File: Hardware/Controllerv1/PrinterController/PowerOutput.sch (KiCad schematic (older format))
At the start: 33 parts, among them J3 Conn_01x03, J4 Conn_01x03, J5 Screw_Terminal_01x08, Q1 Q_NMOS_DGS, Q2 Q_NMOS_DGS, Q3 Q_NMOS_DGS, Q4 Q_NMOS_DGS, Q5 Q_NMOS_DGS, Q6 Q_NMOS_DGS, U2 ZXGD3003E6, U3 ZXGD3003E6, U4 ZXGD3003E6, U5 ZXGD3003E6, U6 ZXGD3003E6, U7 ZXGD3003E6

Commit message: Added updates to PCB
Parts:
- removed Q1, Q2, Q3, Q4: Q_NMOS_DGS, .pretty:SOT65P330X90-5N, symbol Q_NMOS_DGS
- added U10, U11, U8, U9: IRFR3711TRPBF, IRFR3711TRPBF:TO252, symbol IRFR3711TRPBF
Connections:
- net labels removed: VDC
- wire segments 75 -> 81

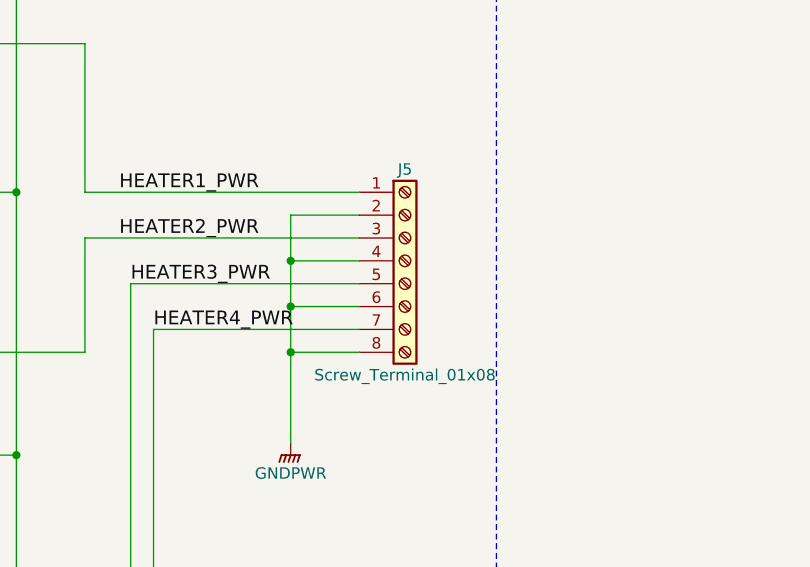
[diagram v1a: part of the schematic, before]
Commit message: Updated PCBS
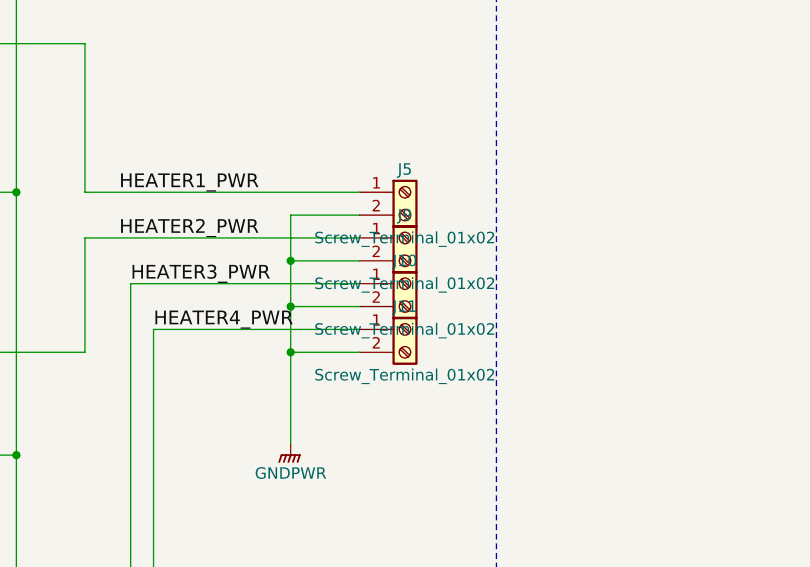
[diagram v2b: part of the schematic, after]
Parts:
- removed J5: Screw_Terminal_01x08, TerminalBlocks_WAGO:TerminalBlock_WAGO-804_RM5mm_8pol, symbol Screw_Terminal_01x08
- added J10, J11, J5, J9: Screw_Terminal_01x02, TerminalBlocks_Phoenix:TerminalBlock_Phoenix_PT-3.5mm_2pol, symbol Screw_Terminal_01x02
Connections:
- net GNDPWR: now also J10.2 (Pin_2), J11.2 (Pin_2), J5.2 (Pin_2), J9.2 (Pin_2)
- net HEATER1_PWR: now also J5.1 (Pin_1)
- net HEATER2_PWR: now also J9.1 (Pin_1)
- net HEATER3_PWR: now also J10.1 (Pin_1)
- net HEATER4_PWR: now also J11.1 (Pin_1)
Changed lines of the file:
@@
 Connection ~ 4050 2450
 $Comp
-L +VDC #PWR077
+L +VDC #PWR083
 U 1 1 5B23E478
 P 4050 1350
-F 0 "#PWR077" H 4050 1250 50  0001 C CNN
+F 0 "#PWR083" H 4050 1250 50  0001 C CNN
 F 1 "+VDC" H 4050 1600 50  0000 C CNN
 F 2 "" H 4050 1350 50  0001 C CNN
@@
 $EndComp
 $Comp
-L Screw_Terminal_01x08 J5
-U 1 1 5B23E5D0
-P 5750 2750
-F 0 "J5" H 5750 3150 50  0000 C CNN
-F 1 "Screw_Terminal_01x08" H 5750 2250 50  0000 C CNN
-F 2 "TerminalBlocks_WAGO:TerminalBlock_WAGO-804_RM5mm_8pol" H 5750 2750 50  0001 C CNN
-F 3 "" H 5750 2750 50  0001 C CNN
-	1    5750 2750
-	1    0    0    -1
-$EndComp
-$Comp
-L GND #PWR078
+L GND #PWR084
 U 1 1 5B23EDD4
 P 2150 1850
-F 0 "#PWR078" H 2150 1600 50  0001 C CNN
+F 0 "#PWR084" H 2150 1600 50  0001 C CNN
 F 1 "GND" H 2150 1700 50  0000 C CNN
 F 2 "" H 2150 1850 50  0001 C CNN
@@
 Connection ~ 4050 1350
 $Comp
-L GNDPWR #PWR079
+L GNDPWR #PWR085
 U 1 1 5B23F80C
 P 5250 3550
-F 0 "#PWR079" H 5250 3350 50  0001 C CNN
+F 0 "#PWR085" H 5250 3350 50  0001 C CNN
 F 1 "GNDPWR" H 5250 3420 50  0000 C CNN
 F 2 "" H 5250 3500 50  0001 C CNN
@@
 $EndComp
 $Comp
-L GND #PWR080
+L GND #PWR086
 U 1 1 5B240503
 P 2150 2950
-F 0 "#PWR080" H 2150 2700 50  0001 C CNN
+F 0 "#PWR086" H 2150 2700 50  0001 C CNN
 F 1 "GND" H 2150 2800 50  0000 C CNN
 F 2 "" H 2150 2950 50  0001 C CNN
@@
 $EndComp
 $Comp
-L GND #PWR081
+L GND #PWR087
 U 1 1 5B240680
 P 2200 4100
-F 0 "#PWR081" H 2200 3850 50  0001 C CNN
+F 0 "#PWR087" H 2200 3850 50  0001 C CNN
 F 1 "GND" H 2200 3950 50  0000 C CNN
 F 2 "" H 2200 4100 50  0001 C CNN
@@
 $EndComp
 $Comp
-L GND #PWR082
+L GND #PWR088
 U 1 1 5B2409DB
 P 2250 5250
-F 0 "#PWR082" H 2250 5000 50  0001 C CNN
+F 0 "#PWR088" H 2250 5000 50  0001 C CNN
 F 1 "GND" H 2250 5100 50  0000 C CNN
 F 2 "" H 2250 5250 50  0001 C CNN
@@
 	3500 6000 3500 6100
 $Comp
-L GNDPWR #PWR083
+L GNDPWR #PWR089
 U 1 1 5B24648A
 P 5050 5950
-F 0 "#PWR083" H 5050 5750 50  0001 C CNN
+F 0 "#PWR089" H 5050 5750 50  0001 C CNN
 F 1 "GNDPWR" H 5050 5820 50  0000 C CNN
 F 2 "" H 5050 5900 50  0001 C CNN
@@
 $EndComp
 $Comp
-L GNDPWR #PWR084
+L GNDPWR #PWR090
 U 1 1 5B246513
 P 5050 6700
-F 0 "#PWR084" H 5050 6500 50  0001 C CNN
+F 0 "#PWR090" H 5050 6500 50  0001 C CNN
 F 1 "GNDPWR" H 5050 6570 50  0000 C CNN
 F 2 "" H 5050 6650 50  0001 C CNN
@@
 $EndComp
 $Comp
-L GND #PWR085
+L GND #PWR091
 U 1 1 5B2466C8
 P 2250 6350
-F 0 "#PWR085" H 2250 6100 50  0001 C CNN
+F 0 "#PWR091" H 2250 6100 50  0001 C CNN
 F 1 "GND" H 2250 6200 50  0000 C CNN
 F 2 "" H 2250 6350 50  0001 C CNN
@@
 $EndComp
 $Comp
-L GND #PWR086
+L GND #PWR092
 U 1 1 5B2469E1
 P 2250 7450
-F 0 "#PWR086" H 2250 7200 50  0001 C CNN
+F 0 "#PWR092" H 2250 7200 50  0001 C CNN
 F 1 "GND" H 2250 7300 50  0000 C CNN
 F 2 "" H 2250 7450 50  0001 C CNN
@@
 	1700 3800 1700 3700
 $Comp
-L GND #PWR087
+L GND #PWR093
 U 1 1 5B248152
 P 6900 1300
-F 0 "#PWR087" H 6900 1050 50  0001 C CNN
+F 0 "#PWR093" H 6900 1050 50  0001 C CNN
 F 1 "GND" H 6900 1150 50  0000 C CNN
 F 2 "" H 6900 1300 50  0001 C CNN
@@
 $EndComp
 $Comp
-L GND #PWR088
+L GND #PWR094
 U 1 1 5B2481C7
 P 7200 1300
-F 0 "#PWR088" H 7200 1050 50  0001 C CNN
+F 0 "#PWR094" H 7200 1050 50  0001 C CNN
 F 1 "GND" H 7200 1150 50  0000 C CNN
 F 2 "" H 7200 1300 50  0001 C CNN
@@
 $EndComp
 $Comp
-L GND #PWR089
+L GND #PWR095
 U 1 1 5B248235
 P 7500 1300
-F 0 "#PWR089" H 7500 1050 50  0001 C CNN
+F 0 "#PWR095" H 7500 1050 50  0001 C CNN
 F 1 "GND" H 7500 1150 50  0000 C CNN
 F 2 "" H 7500 1300 50  0001 C CNN
@@
 $EndComp
 $Comp
-L GND #PWR090
+L GND #PWR096
 U 1 1 5B2482A3
 P 7800 1300
-F 0 "#PWR090" H 7800 1050 50  0001 C CNN
+F 0 "#PWR096" H 7800 1050 50  0001 C CNN
 F 1 "GND" H 7800 1150 50  0000 C CNN
 F 2 "" H 7800 1300 50  0001 C CNN
@@
 $EndComp
 $Comp
-L GND #PWR091
+L GND #PWR097
 U 1 1 5B248311
 P 8150 1300
-F 0 "#PWR091" H 8150 1050 50  0001 C CNN
+F 0 "#PWR097" H 8150 1050 50  0001 C CNN
 F 1 "GND" H 8150 1150 50  0000 C CNN
 F 2 "" H 8150 1300 50  0001 C CNN
@@
 $EndComp
 $Comp
-L GND #PWR092
+L GND #PWR098
 U 1 1 5B24837F
 P 8550 1300
-F 0 "#PWR092" H 8550 1050 50  0001 C CNN
+F 0 "#PWR098" H 8550 1050 50  0001 C CNN
 F 1 "GND" H 8550 1150 50  0000 C CNN
 F 2 "" H 8550 1300 50  0001 C CNN
@@
 	3600 1800 3600 1650
 $Comp
-L +VDC #PWR093
+L +VDC #PWR099
 U 1 1 5B262DD2
 P 6900 1000
-F 0 "#PWR093" H 6900 900 50  0001 C CNN
+F 0 "#PWR099" H 6900 900 50  0001 C CNN
 F 1 "+VDC" H 6900 1250 50  0000 C CNN
 F 2 "" H 6900 1000 50  0001 C CNN
@@
 $EndComp
 $Comp
-L +VDC #PWR094
+L +VDC #PWR0100
 U 1 1 5B262E40
 P 7200 1000
-F 0 "#PWR094" H 7200 900 50  0001 C CNN
+F 0 "#PWR0100" H 7200 900 50  0001 C CNN
 F 1 "+VDC" H 7200 1250 50  0000 C CNN
 F 2 "" H 7200 1000 50  0001 C CNN
@@
 $EndComp
 $Comp
-L +VDC #PWR095
+L +VDC #PWR0101
 U 1 1 5B262EAE
 P 7500 1000
-F 0 "#PWR095" H 7500 900 50  0001 C CNN
+F 0 "#PWR0101" H 7500 900 50  0001 C CNN
 F 1 "+VDC" H 7500 1250 50  0000 C CNN
 F 2 "" H 7500 1000 50  0001 C CNN
@@
 $EndComp
 $Comp
-L +VDC #PWR096
+L +VDC #PWR0102
 U 1 1 5B262F1C
 P 7800 1000
-F 0 "#PWR096" H 7800 900 50  0001 C CNN
+F 0 "#PWR0102" H 7800 900 50  0001 C CNN
 F 1 "+VDC" H 7800 1250 50  0000 C CNN
 F 2 "" H 7800 1000 50  0001 C CNN
@@
 $EndComp
 $Comp
-L +VDC #PWR097
+L +VDC #PWR0103
 U 1 1 5B262F8A
 P 8150 1000
-F 0 "#PWR097" H 8150 900 50  0001 C CNN
+F 0 "#PWR0103" H 8150 900 50  0001 C CNN
 F 1 "+VDC" H 8150 1250 50  0000 C CNN
 F 2 "" H 8150 1000 50  0001 C CNN
@@
 $EndComp
 $Comp
-L +VDC #PWR098
+L +VDC #PWR0104
 U 1 1 5B262FF8
 P 8550 1000
-F 0 "#PWR098" H 8550 900 50  0001 C CNN
+F 0 "#PWR0104" H 8550 900 50  0001 C CNN
 F 1 "+VDC" H 8550 1250 50  0000 C CNN
 F 2 "" H 8550 1000 50  0001 C CNN
@@
 $EndComp
 $Comp
-L +VDC #PWR099
+L +VDC #PWR0105
 U 1 1 5B263066
 P 2150 1250
-F 0 "#PWR099" H 2150 1150 50  0001 C CNN
+F 0 "#PWR0105" H 2150 1150 50  0001 C CNN
 F 1 "+VDC" H 2150 1500 50  0000 C CNN
 F 2 "" H 2150 1250 50  0001 C CNN
@@
 $EndComp
 $Comp
-L +VDC #PWR0100
+L +VDC #PWR0106
 U 1 1 5B2630F5
 P 2150 2350
-F 0 "#PWR0100" H 2150 2250 50  0001 C CNN
+F 0 "#PWR0106" H 2150 2250 50  0001 C CNN
 F 1 "+VDC" H 2150 2600 50  0000 C CNN
 F 2 "" H 2150 2350 50  0001 C CNN
@@
 $EndComp
 $Comp
-L +VDC #PWR0101
+L +VDC #PWR0107
 U 1 1 5B263163
 P 2200 3500
-F 0 "#PWR0101" H 2200 3400 50  0001 C CNN
+F 0 "#PWR0107" H 2200 3400 50  0001 C CNN
 F 1 "+VDC" H 2200 3750 50  0000 C CNN
 F 2 "" H 2200 3500 50  0001 C CNN
@@
 $EndComp
 $Comp
-L +VDC #PWR0102
+L +VDC #PWR0108
 U 1 1 5B2631D1
 P 2250 4650
-F 0 "#PWR0102" H 2250 4550 50  0001 C CNN
+F 0 "#PWR0108" H 2250 4550 50  0001 C CNN
 F 1 "+VDC" H 2250 4900 50  0000 C CNN
 F 2 "" H 2250 4650 50  0001 C CNN
@@
 $EndComp
 $Comp
-L +VDC #PWR0103
+L +VDC #PWR0109
 U 1 1 5B2632C3
 P 2250 5750
-F 0 "#PWR0103" H 2250 5650 50  0001 C CNN
+F 0 "#PWR0109" H 2250 5650 50  0001 C CNN
 F 1 "+VDC" H 2250 6000 50  0000 C CNN
 F 2 "" H 2250 5750 50  0001 C CNN
@@
 $EndComp
 $Comp
-L +VDC #PWR0104
+L +VDC #PWR0110
 U 1 1 5B2633E6
 P 2250 6850
-F 0 "#PWR0104" H 2250 6750 50  0001 C CNN
+F 0 "#PWR0110" H 2250 6750 50  0001 C CNN
 F 1 "+VDC" H 2250 7100 50  0000 C CNN
 F 2 "" H 2250 6850 50  0001 C CNN
@@
 	1    0    0    -1
 $EndComp
+$Comp
+L Screw_Terminal_01x02 J5
+U 1 1 5B32BB01
+P 5750 2450
+F 0 "J5" H 5750 2550 50  0000 C CNN
+F 1 "Screw_Terminal_01x02" H 5750 2250 50  0000 C CNN
+F 2 "TerminalBlocks_Phoenix:TerminalBlock_Phoenix_PT-3.5mm_2pol" H 5750 2450 50  0001 C CNN
+F 3 "" H 5750 2450 50  0001 C CNN
+	1    5750 2450
+	1    0    0    -1
+$EndComp
+$Comp
+L Screw_Terminal_01x02 J9
+U 1 1 5B32BB8B
+P 5750 2650
+F 0 "J9" H 5750 2750 50  0000 C CNN
+F 1 "Screw_Terminal_01x02" H 5750 2450 50  0000 C CNN
+F 2 "TerminalBlocks_Phoenix:TerminalBlock_Phoenix_PT-3.5mm_2pol" H 5750 2650 50  0001 C CNN
+F 3 "" H 5750 2650 50  0001 C CNN
+	1    5750 2650
+	1    0    0    -1
+$EndComp
+$Comp
+L Screw_Terminal_01x02 J10
+U 1 1 5B32BC79
+P 5750 2850
+F 0 "J10" H 5750 2950 50  0000 C CNN
+F 1 "Screw_Terminal_01x02" H 5750 2650 50  0000 C CNN
+F 2 "TerminalBlocks_Phoenix:TerminalBlock_Phoenix_PT-3.5mm_2pol" H 5750 2850 50  0001 C CNN
+F 3 "" H 5750 2850 50  0001 C CNN
+	1    5750 2850
+	1    0    0    -1
+$EndComp
+$Comp
+L Screw_Terminal_01x02 J11
+U 1 1 5B32BCFA
+P 5750 3050
+F 0 "J11" H 5750 3150 50  0000 C CNN
+F 1 "Screw_Terminal_01x02" H 5750 2850 50  0000 C CNN
+F 2 "TerminalBlocks_Phoenix:TerminalBlock_Phoenix_PT-3.5mm_2pol" H 5750 3050 50  0001 C CNN
+F 3 "" H 5750 3050 50  0001 C CNN
+	1    5750 3050
+	1    0    0    -1
+$EndComp

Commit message: Added routed Power switching circuitry
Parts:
- removed R16, R18: 10k, Resistors_SMD:R_0805, symbol R
- removed U6, U7: ZXGD3003E6, TO_SOT_Packages_SMD:SOT-23-6, symbol ZXGD3003E6
- added D4, D5: D, Diodes_SMD:D_SOD-123, symbol Device:D
- added JP1, JP2: Jumper_NC_Small, Pin_Headers:Pin_Header_Straight_1x02_Pitch2.54mm, symbol Device:Jumper_NC_Small
- C27, C28, C29, C30, C31, C32: symbol CP -> PrinterController-rescue:CP
- J10, J11, J5, J9: symbol Screw_Terminal_01x02 -> PrinterController-rescue:Screw_Terminal_01x02
- J3, J4: symbol Conn_01x03 -> PrinterController-rescue:Conn_01x03
- Q5, Q6: symbol Q_NMOS_DGS -> PrinterController-rescue:Q_NMOS_DGS
- R10, R11, R12, R13, R14, R15, R17, R7, R8, R9: symbol R -> PrinterController-rescue:R
- U10, U11, U8, U9: symbol IRFR3711TRPBF -> PrinterController-rescue:IRFR3711TRPBF
- U2, U3, U4, U5: symbol ZXGD3003E6 -> PrinterController-rescue:ZXGD3003E6
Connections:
- net labels added: +5V
- net labels removed: GND
- wire segments 81 -> 94
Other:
- moved on the sheet: C31, C32, R15, R17

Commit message: Added updates to controller hardware
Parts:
- C27, C28, C29, C30, C31, C32: footprint Capacitors_Tantalum_SMD:CP_Tantalum_Case-A_EIA-3216-18_Hand -> Capacitors_SMD:CP_Elec_6.3x5.3
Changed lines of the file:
@@
 F 0 "C27" H 6925 1250 50  0000 L CNN
 F 1 "47u" H 6925 1050 50  0000 L CNN
-F 2 "Capacitors_Tantalum_SMD:CP_Tantalum_Case-A_EIA-3216-18_Hand" H 6938 1000 50  0001 C CNN
+F 2 "Capacitors_SMD:CP_Elec_6.3x5.3" H 6938 1000 50  0001 C CNN
 F 3 "" H 6900 1150 50  0001 C CNN
 	1    6900 1150
@@
 F 0 "C28" H 7225 1250 50  0000 L CNN
 F 1 "47u" H 7225 1050 50  0000 L CNN
-F 2 "Capacitors_Tantalum_SMD:CP_Tantalum_Case-A_EIA-3216-18_Hand" H 7238 1000 50  0001 C CNN
+F 2 "Capacitors_SMD:CP_Elec_6.3x5.3" H 7238 1000 50  0001 C CNN
 F 3 "" H 7200 1150 50  0001 C CNN
 	1    7200 1150
@@
 F 0 "C29" H 7525 1250 50  0000 L CNN
 F 1 "47u" H 7525 1050 50  0000 L CNN
-F 2 "Capacitors_Tantalum_SMD:CP_Tantalum_Case-A_EIA-3216-18_Hand" H 7538 1000 50  0001 C CNN
+F 2 "Capacitors_SMD:CP_Elec_6.3x5.3" H 7538 1000 50  0001 C CNN
 F 3 "" H 7500 1150 50  0001 C CNN
 	1    7500 1150
@@
 F 0 "C30" H 7825 1250 50  0000 L CNN
 F 1 "47u" H 7825 1050 50  0000 L CNN
-F 2 "Capacitors_Tantalum_SMD:CP_Tantalum_Case-A_EIA-3216-18_Hand" H 7838 1000 50  0001 C CNN
+F 2 "Capacitors_SMD:CP_Elec_6.3x5.3" H 7838 1000 50  0001 C CNN
 F 3 "" H 7800 1150 50  0001 C CNN
 	1    7800 1150
@@
 F 0 "C31" H 2325 6750 50  0000 L CNN
 F 1 "47u" H 2325 6550 50  0000 L CNN
-F 2 "Capacitors_Tantalum_SMD:CP_Tantalum_Case-A_EIA-3216-18_Hand" H 2338 6500 50  0001 C CNN
+F 2 "Capacitors_SMD:CP_Elec_6.3x5.3" H 2338 6500 50  0001 C CNN
 F 3 "" H 2300 6650 50  0001 C CNN
 	1    2300 6650
@@
 F 0 "C32" H 2725 6750 50  0000 L CNN
 F 1 "47u" H 2725 6550 50  0000 L CNN
-F 2 "Capacitors_Tantalum_SMD:CP_Tantalum_Case-A_EIA-3216-18_Hand" H 2738 6500 50  0001 C CNN
+F 2 "Capacitors_SMD:CP_Elec_6.3x5.3" H 2738 6500 50  0001 C CNN
 F 3 "" H 2700 6650 50  0001 C CNN
 	1    2700 6650
